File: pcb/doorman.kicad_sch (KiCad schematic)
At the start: 42 parts, among them J1 USB_C_Receptacle_USB2.0, J2 Terminal, J3 3V3 Test Pad, J4 Conn_02x07_Odd_Even, J6 BUS Test Pad, J7 BUS RX Test Pad, J8 TX Test Pad, J9 RX Test Pad, Q1 BC847BPN, Q2 BC817, SW1 Reset Button, SW2 Flash Button, U2 AP63203WU, U3 GAQY252G3S, U4 ESP32-S3-MINI-1

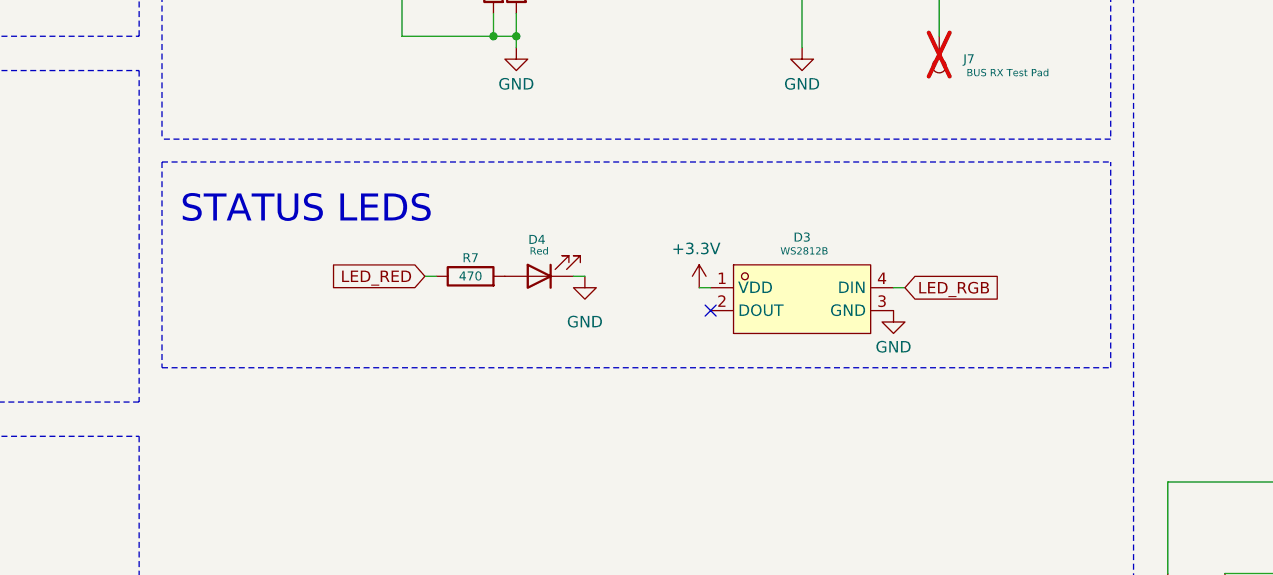
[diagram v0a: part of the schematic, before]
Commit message: WIP
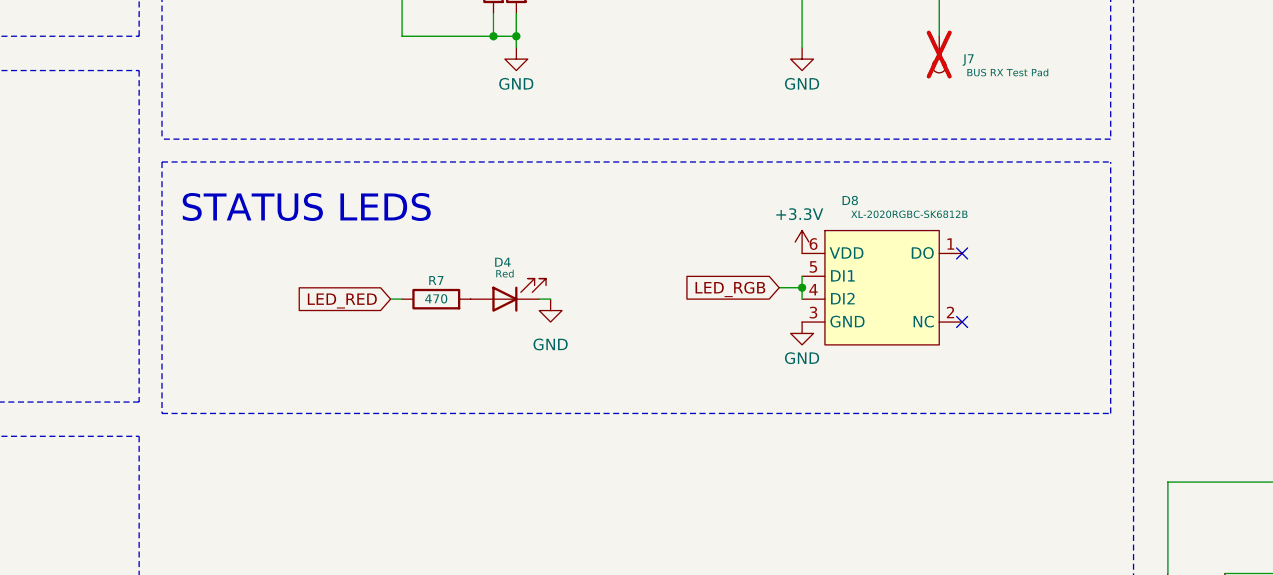
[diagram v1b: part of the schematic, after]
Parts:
- removed D3: WS2812B, Doorman:LED-SMD_4P-L2.0-W1.8_CY-0807, symbol easyeda2kicad:XL-0807RGBC-WS2812B
- added D8: XL-2020RGBC-SK6812B, Doorman:LED-SMD_6P-L2.0-W2.0_XL-2020RGBC, symbol easyeda2kicad:XL-2020RGBC-SK6812B
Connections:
- net +3.3V: now also D8.6 (VDD)
- net GND: now also D8.3 (GND)
- net LED_RGB: now also D8.4 (DI2), D8.5 (DI1)
- no-connect marks 21 -> 22
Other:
- moved on the sheet: D4, R7

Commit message: WIP
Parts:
- D8: LCSC (none) -> C5349956; MPN (none) -> XL-2020RGBC-SK6812B; Package (none) -> 2020
- R11, R8: LCSC C2933356 -> C5140149; MPN FRC0805F1R20TS -> SCR0805J1R2
- R12, R6: LCSC C22878 -> C25804; MPN 0603WAF1473T5E -> 0603WAF1002T5E
- R5: LCSC C22935 -> C25819; MPN 0603WAF1004T5E -> 0603WAF4702T5E
